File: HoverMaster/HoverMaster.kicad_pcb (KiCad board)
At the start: 2 copper layers, 199.6 x 35 mm, 14 parts, among them J1 Conn_01x02_Male, J2 Conn_01x03_Male, J3 Conn_01x04_Male, J4 Conn_01x09, J5 Conn_01x03, J6 Conn_01x03, J7 Conn_01x03_Male, J8 Conn_01x03_Male, SW1 SW_Push, U1 NodeMCU_Amica_R2

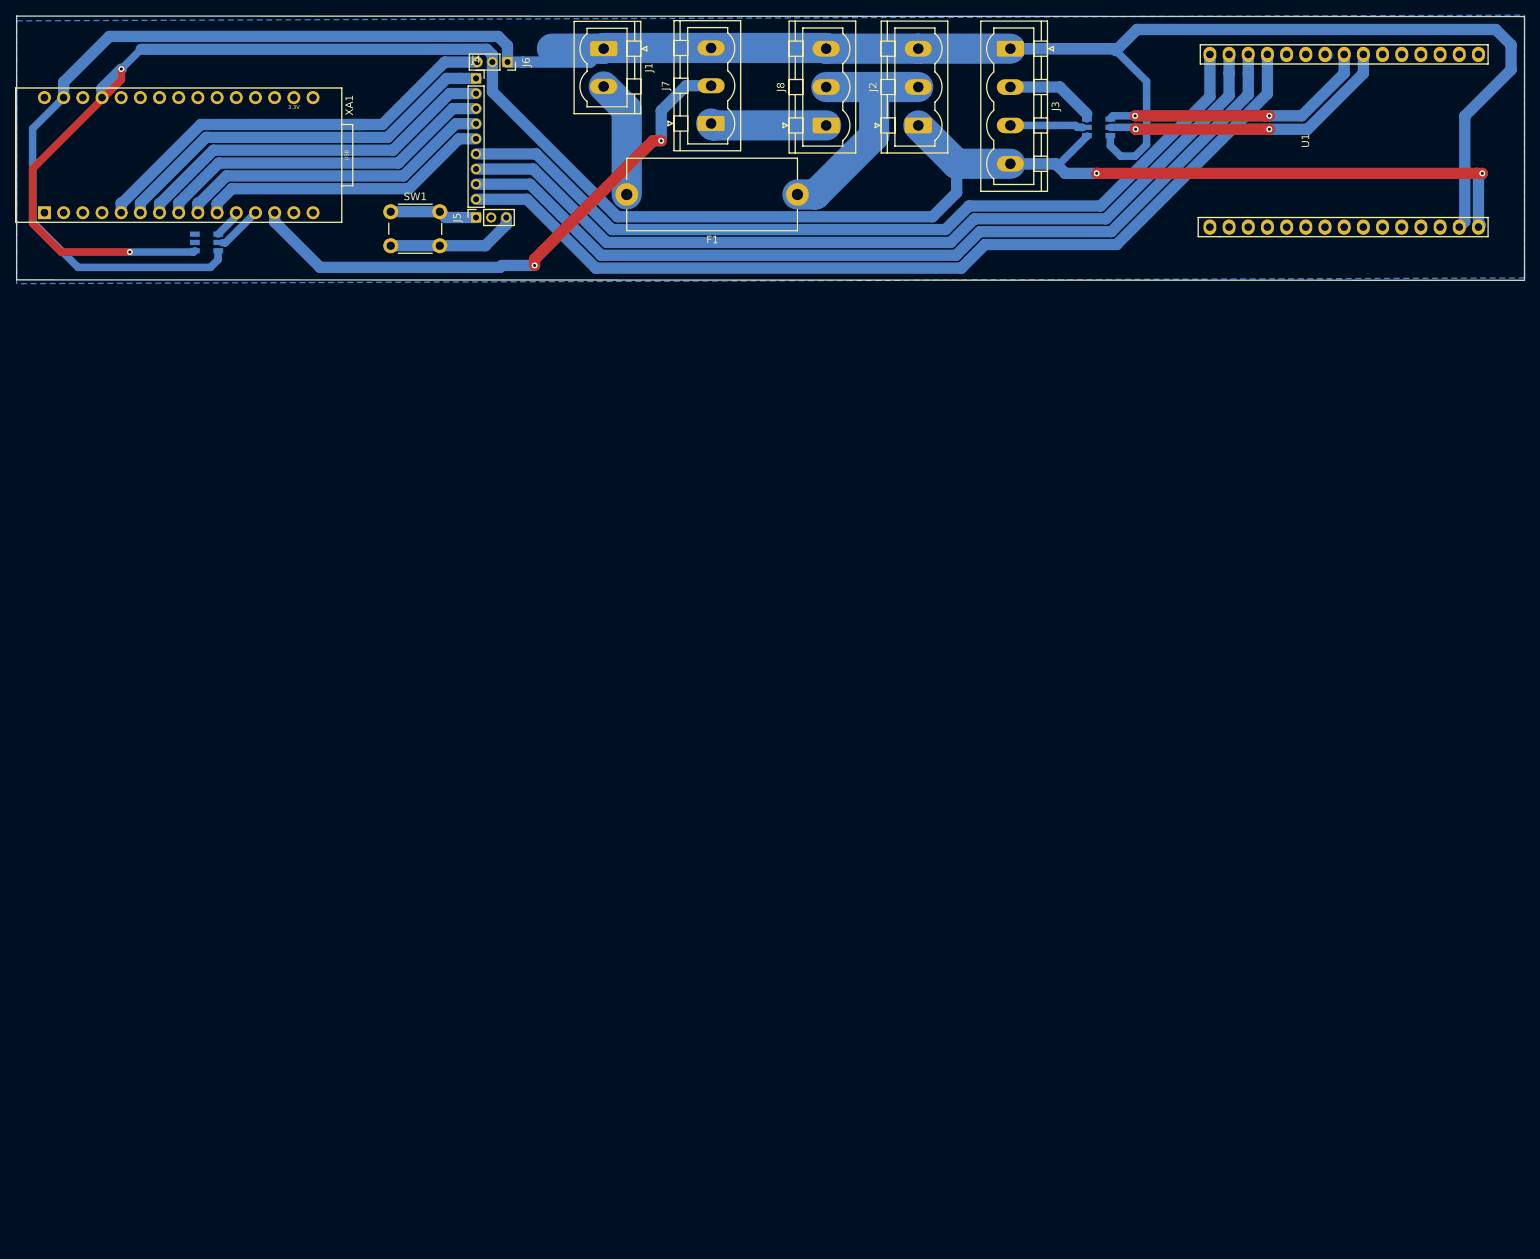
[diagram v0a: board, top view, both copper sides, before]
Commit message: hovermaster
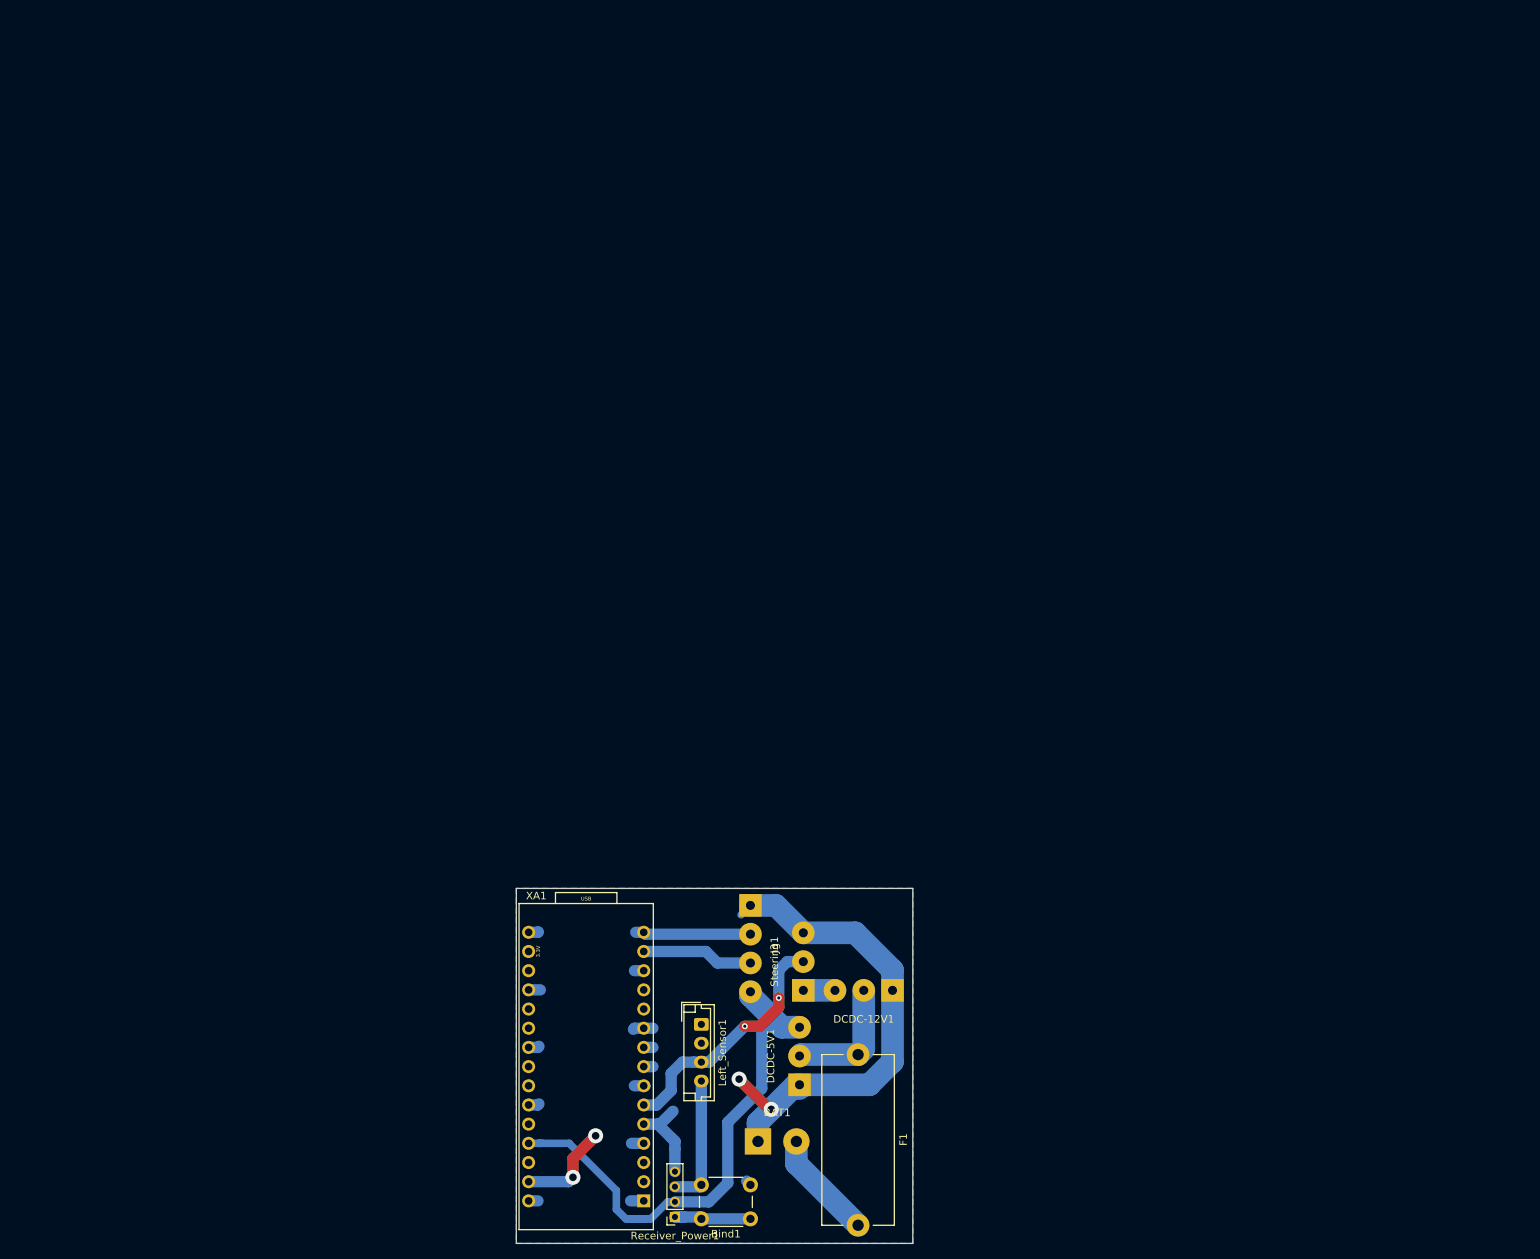
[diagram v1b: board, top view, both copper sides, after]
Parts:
- removed D1, D2: APA102, LED_SMD:LED_RGB_PLCC-6
- removed J1: Conn_01x02_Male, Connector_Phoenix_MSTB:PhoenixContact_MSTBVA_2,5_2-G_1x02_P5.00mm_Vertical
- removed J2, J8: Conn_01x03_Male, Connector_Phoenix_MSTB:PhoenixContact_MSTBVA_2,5_3-G-5,08_1x03_P5.08mm_Vertical
- removed J4: Conn_01x09, Connector_PinSocket_2.00mm:PinSocket_1x09_P2.00mm_Vertical
- removed J5, J6: Conn_01x03, Connector_PinSocket_2.00mm:PinSocket_1x03_P2.00mm_Vertical
- removed J7: Conn_01x03_Male, Connector_Phoenix_MSTB:PhoenixContact_MSTBVA_2,5_3-G_1x03_P5.00mm_Vertical
- removed SW1: SW_Push, Button_Switch_THT:SW_PUSH_6mm
- removed U1: NodeMCU_Amica_R2, nodemcu:NodeMCU_Amica_R2
- added BAT1: Conn_01x02_Male, Connector_Wire:SolderWirePad_1x02_P5.08mm_Drill1.5mm, F.Cu at (104.0, 149.0)
- added Bind1: SW_Push, Button_Switch_THT:SW_PUSH_6mm, F.Cu at (103.0, 159.2)
- added DCDC-12V1: DCDC-12V, Connector_Wire:SolderWirePad_1x03_P3.81mm_Drill1.2mm, F.Cu at (121.8, 129.0)
- added DCDC-5V1: Conn_01x03_Male, Connector_Wire:SolderWirePad_1x03_P3.81mm_Drill1.2mm, F.Cu at (109.5, 141.5)
- added Left_Sensor1: Conn_01x04, Connector_JST:JST_EH_B4B-EH-A_1x04_P2.50mm_Vertical, F.Cu at (96.5, 133.5)
- added Receiver_Power1: Conn_01x04, Connector_PinSocket_2.00mm:PinSocket_1x04_P2.00mm_Vertical, F.Cu at (93.0, 159.0)
- added Steering1: Conn_01x03_Male, Connector_Wire:SolderWirePad_1x03_P3.81mm_Drill1.2mm, F.Cu at (110.0, 129.0)
- J3: value Conn_01x04_Male -> LED; footprint Connector_Phoenix_MSTB:PhoenixContact_MSTBVA_2,5_4-G-5,08_1x04_P5.08mm_Vertical -> Connector_Wire:SolderWirePad_1x04_P3.81mm_Drill1.2mm
- moved J3 118.5 mm to (103.0, 117.8)
- moved F1 114.2 mm to (117.2, 137.5), turned to 270 degrees
- moved XA1 104.2 mm to (81.2, 117.5), turned to 180 degrees
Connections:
- XA1 pad 3V3: Net-(XA1-Pad3V3) -> (no net)
- XA1 pad A0: Net-(XA1-PadA0) -> (no net)
- XA1 pad A1: Net-(XA1-PadA1) -> (no net)
- XA1 pad A2: Net-(XA1-PadA2) -> (no net)
- XA1 pad A3: Net-(XA1-PadA3) -> (no net)
- XA1 pad A4: Net-(XA1-PadA4) -> (no net)
- XA1 pad A5: Net-(XA1-PadA5) -> (no net)
- XA1 pad A6: Net-(XA1-PadA6) -> (no net)
- XA1 pad A7: Net-(XA1-PadA7) -> (no net)
- XA1 pad AREF: Net-(XA1-PadAREF) -> (no net)
- XA1 pad D0: Net-(XA1-PadD0) -> (no net)
- XA1 pad D1: Net-(XA1-PadD1) -> (no net)
- XA1 pad D10: Signal_Steering -> (no net)
- XA1 pad D11: Signal_Light -> LED2
- XA1 pad D12: Net-(XA1-PadD12) -> LED1
- XA1 pad D13: Net-(XA1-PadD13) -> (no net)
- XA1 pad D2: C1 -> PPM_IN
- XA1 pad D3: C2 -> PPM_OUT
- XA1 pad D4: C3 -> (no net)
- XA1 pad D5: C4 -> (no net)
- XA1 pad D6: C5 -> (no net)
- XA1 pad D7: C6 -> (no net)
- XA1 pad D8: Status_D -> (no net)
- XA1 pad D9: Status_C -> (no net)
- XA1 pad GND1: Net-(XA1-PadGND1) -> (no net)
- XA1 pad RST1: Net-(XA1-PadRST1) -> (no net)
- XA1 pad RST2: Net-(XA1-PadRST2) -> (no net)
- XA1 pad VIN: Net-(XA1-PadVIN) -> (no net)
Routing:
- net GND: track 317.0 -> 97.2 mm, vias 0 -> 4
- net 5V: track 278.2 -> 70.0 mm, vias 4 -> 0
- net C10: track 123.3 -> 0.00 mm
- net C9: track 120.3 -> 0.00 mm
- net C8: track 117.2 -> 0.00 mm
- net C7: track 114.2 -> 0.00 mm
- net Signal_Steering: track 74.3 -> 0.00 mm, vias 2 -> 0
- net C1: track 57.4 -> 0.00 mm
- net C2: track 52.6 -> 0.00 mm
- net C3: track 49.2 -> 0.00 mm
- net C4: track 45.8 -> 0.00 mm
- net C5: track 42.5 -> 0.00 mm
- net S2: track 39.3 -> 0.00 mm, vias 2 -> 0
- net C6: track 39.1 -> 0.00 mm
- net S1: track 35.9 -> 0.00 mm, vias 2 -> 0
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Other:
- board size 199.6 x 35 mm -> 52.5 x 47 mm
